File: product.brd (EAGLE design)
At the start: 59.7 x 31.8 mm, 38 parts, among them IC1 MCP1703CB, Q2 16MHz, U1 ATSHA204-TSU, U2 USB, U3 DISPLAY

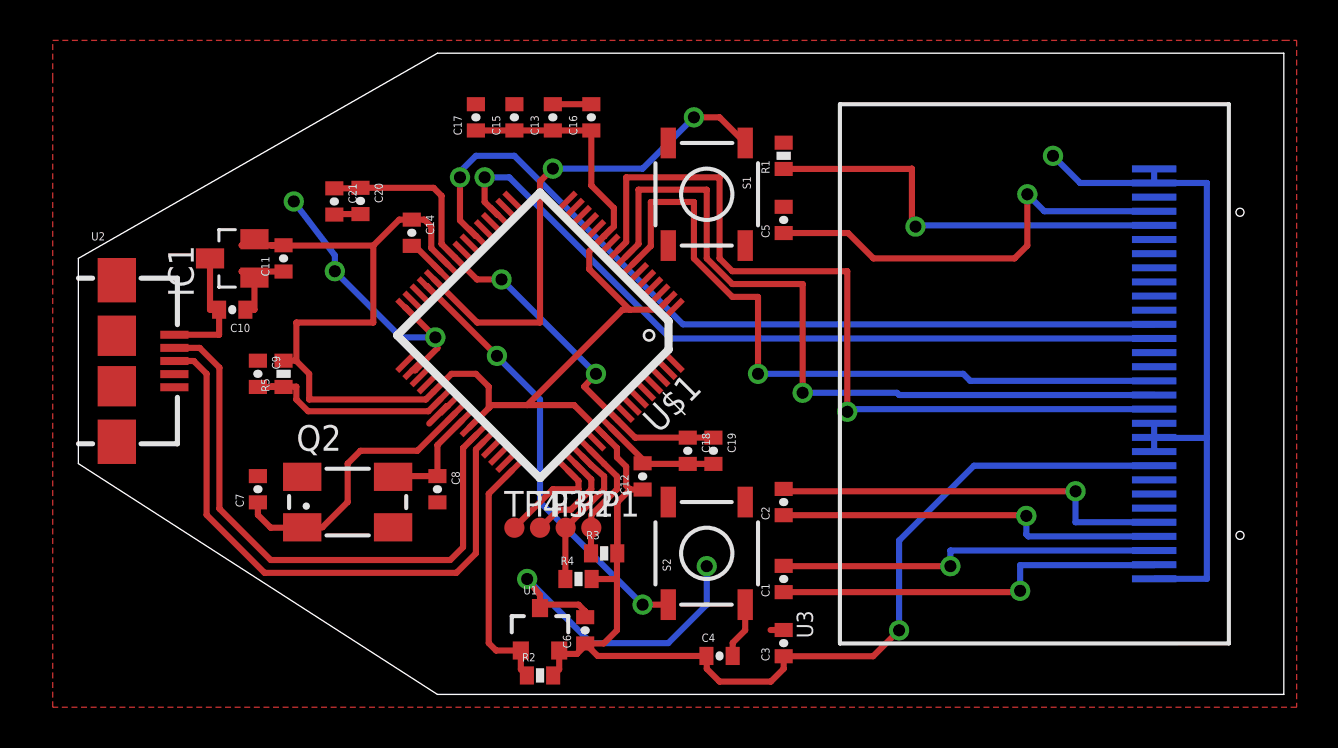
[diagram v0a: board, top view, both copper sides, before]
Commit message: work on pcbs
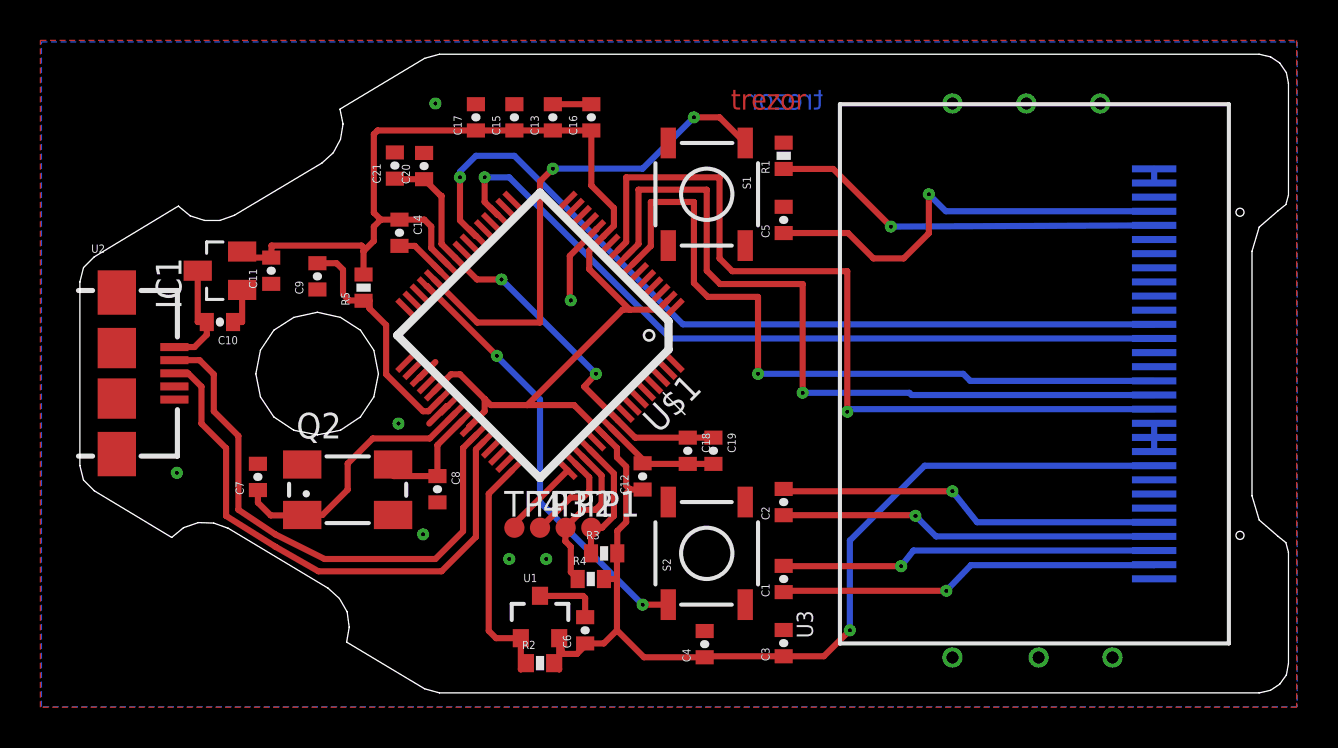
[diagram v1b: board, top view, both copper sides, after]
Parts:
- moved R5 5.82 mm to (14.1, 20.1)
- moved C9 5.65 mm to (11.8, 20.7), turned to 90 degrees
- moved C20 3.59 mm to (17.1, 26.2), turned to 90 degrees
- moved C21 3.48 mm to (15.7, 26.2), turned to 90 degrees
- moved C4 0.94 mm to (31.0, 2.49), turned to 90 degrees
- moved C10 0.86 mm to (7.01, 18.4)
- moved C11 0.86 mm to (9.55, 21.0)
- moved IC1 0.86 mm to (7.01, 21.0)
- moved C14 0.61 mm to (15.9, 22.9)
- moved U2 0.61 mm to (1.91, 15.9)
- moved C7 0.61 mm to (8.89, 10.8)
- moved Q2 0.61 mm to (13.3, 10.1)
- moved R4 0.61 mm to (25.4, 5.71)
- moved U1 0.61 mm to (22.9, 3.78)
- moved R2 0.61 mm to (22.9, 1.55)
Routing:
- net GND: track 88.0 -> 24.3 mm, vias 6 -> 13
- net +3V3: track 126.4 -> 113.1 mm
- net N$23: track 27.1 -> 23.7 mm
- net N$7: track 29.5 -> 27.2 mm
- net N$3: track 28.9 -> 26.9 mm
- net N$9: track 21.1 -> 19.5 mm
- net N$20: track 5.12 -> 3.94 mm
- net +5V: track 6.45 -> 5.48 mm
- net N$13: track 20.0 -> 19.2 mm
- net N$10: track 19.7 -> 18.9 mm
- net N$4: track 35.9 -> 36.7 mm
- net N$21: track 11.4 -> 12.1 mm
- net XTAL1: track 14.1 -> 13.5 mm
- net N$11: track 19.3 -> 18.8 mm
- net XTAL2: track 5.48 -> 6.01 mm
- added copper zone on layer 16, net GND
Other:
- board size 59.7 x 31.8 mm -> 59.8 x 31.6 mm
- board text added: "trezor"
